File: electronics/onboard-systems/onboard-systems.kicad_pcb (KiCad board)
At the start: 2 copper layers, 28.4 x 82.9 mm, 6 parts, among them SW1 GOOBAY_10013, U1 XIAO_ESP32_S3, U2 Adafruit_BMP580, U3 Adafruit_LSM6DSO32

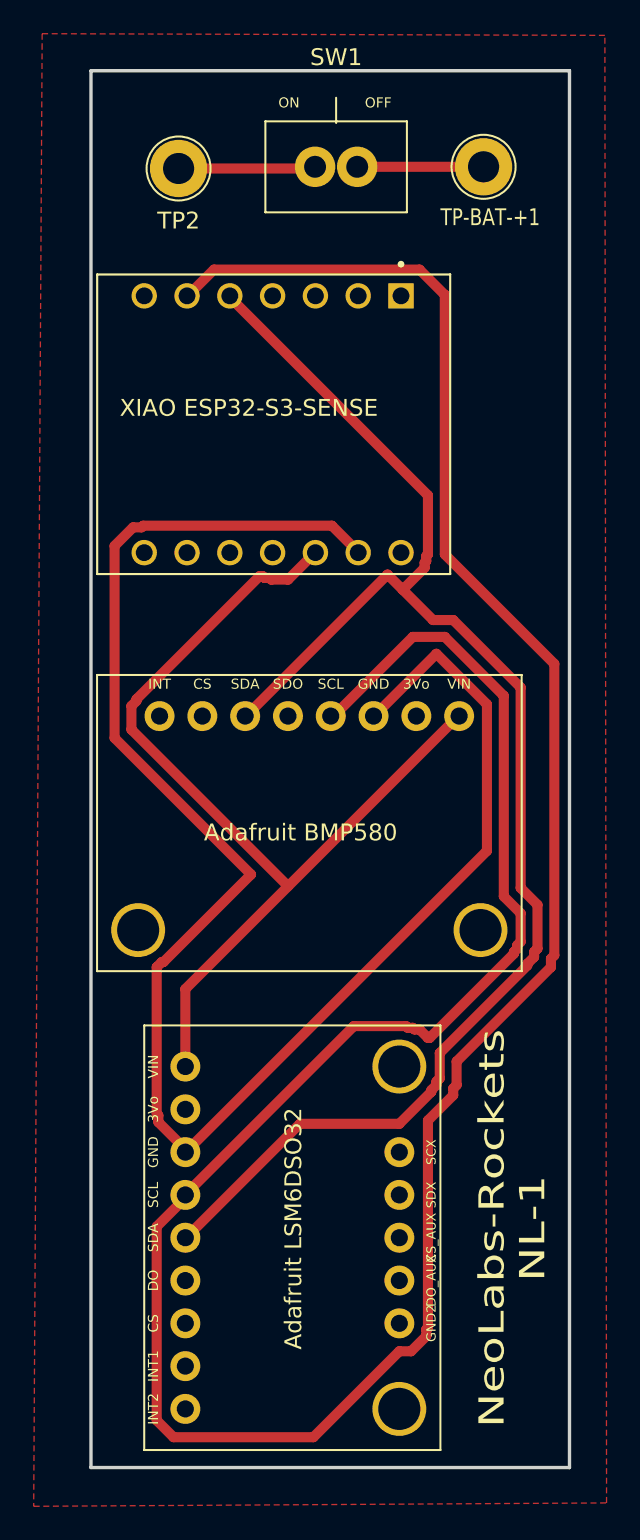
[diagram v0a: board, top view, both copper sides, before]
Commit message: update models
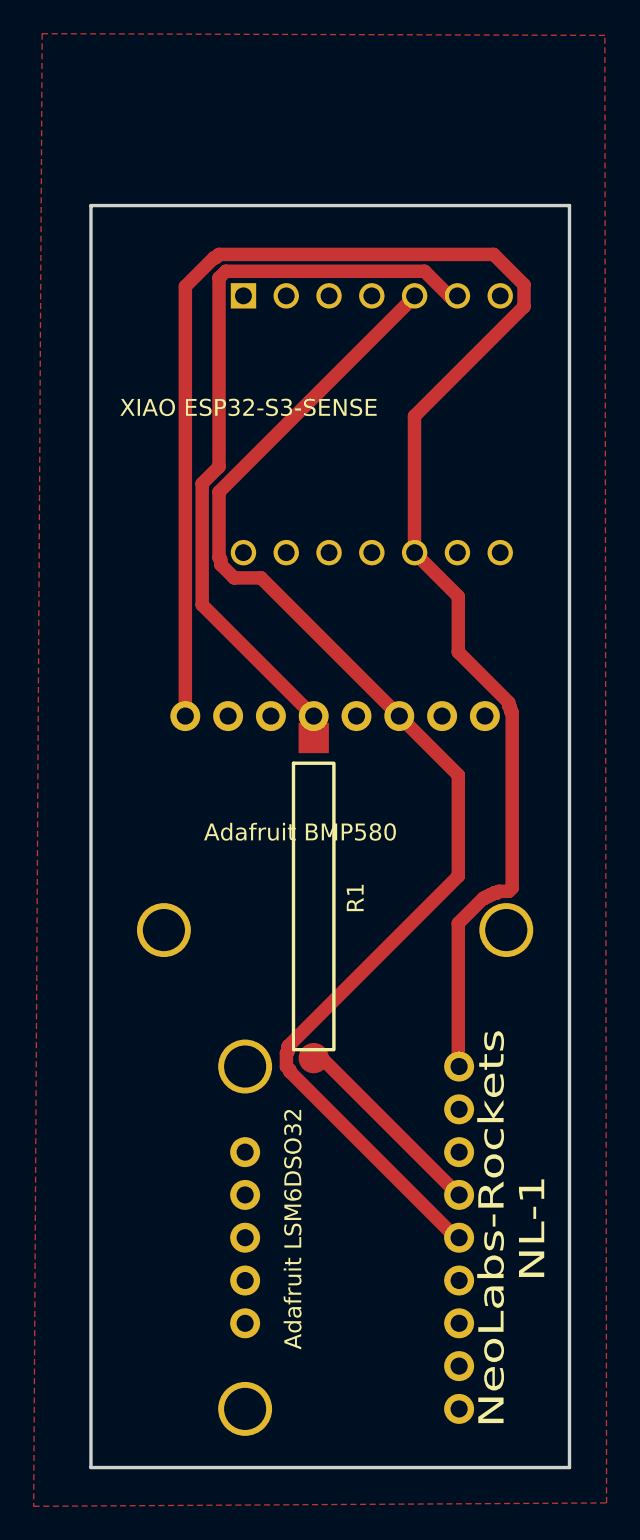
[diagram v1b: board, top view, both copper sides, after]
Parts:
- removed SW1: GOOBAY_10013, GOOBAY:GOOBAY_10013
- removed TP-BAT-+1, TP2: TestPoint, TestPoint:TestPoint_Loop_D2.50mm_Drill1.85mm
- added R1: 0R, Jumper:R_0R_THT_Custom, F.Cu at (166.0, 116.5)
- U1, U2, U3: moved to B.Cu
- moved U1 5.76 mm to (169.4, 88.4)
- moved U3 3.55 mm to (168.3, 136.7)
- moved U2 1.53 mm to (167.3, 112.0), turned to 0 degrees
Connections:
- U3 pad 14: unconnected-(U3-GND2-Pad14) -> GND
- U3 pad 4: Net-(U1-D5/GPIO6) -> SDA_J1_OUT
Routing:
- net Net-(U1-D5/GPIO6): track 172.4 -> 44.0 mm
- net GND: track 101.5 -> 0.00 mm
- net Net-(U1-3V3): track 57.0 -> 100.6 mm
- net Net-(U1-D4/GPIO5): track 90.7 -> 75.9 mm
- net SDA_J1_OUT: track 0.00 -> 12.0 mm
- net Net-(SW1-Pad1): track 8.14 -> 0.00 mm
- net Net-(SW1-Pad2): track 7.50 -> 0.00 mm
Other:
- board size 28.4 x 82.9 mm -> 28.4 x 74.9 mm

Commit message: fix pcb
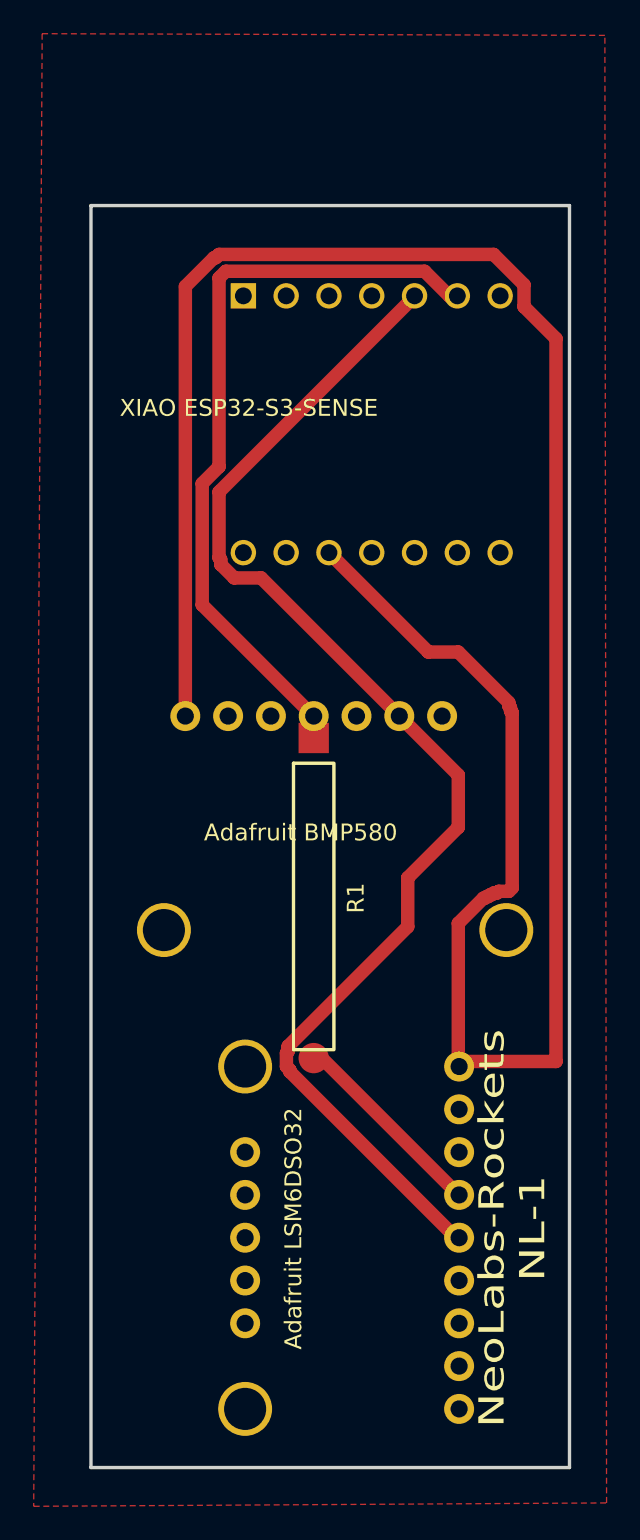
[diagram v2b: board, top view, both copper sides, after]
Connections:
- U3 pad 4: SDA_J1_OUT -> Net-(U1-D5/GPIO6)
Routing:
- net Net-(U1-3V3): track 100.6 -> 137.9 mm
